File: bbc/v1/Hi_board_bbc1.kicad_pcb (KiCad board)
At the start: 2 copper layers, 55 x 61.1 mm, 15 parts, among them J1 sw-latch, J2 led-latch, J3 GLVMP, SW1 BSPD_RESET, SW2 IMD_RESET, SW3 BMS_RESET

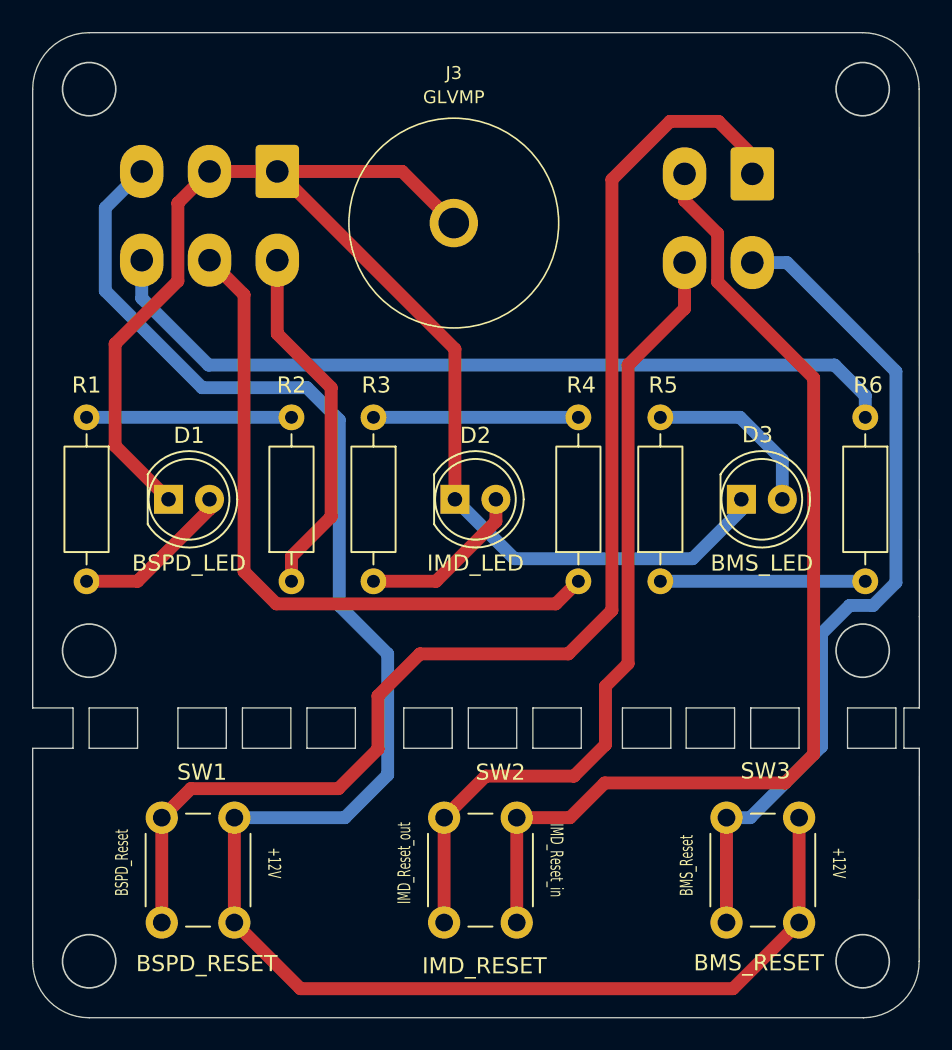
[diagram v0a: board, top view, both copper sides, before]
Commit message: Add files via upload
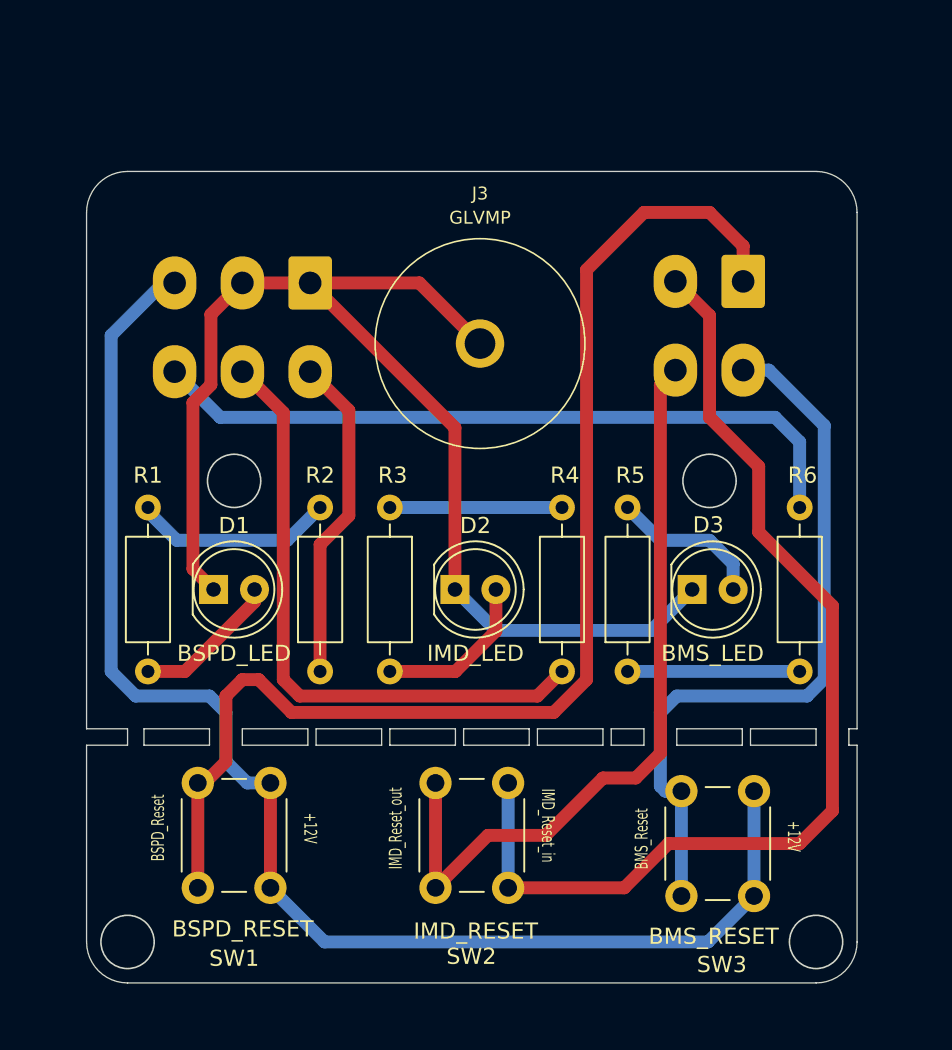
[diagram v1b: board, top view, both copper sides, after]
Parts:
- moved J3 7.64 mm to (141.2, 112.3)
- moved J2 7.20 mm to (130.7, 108.5)
- moved R6 6.91 mm to (161.0, 122.4)
- moved R1 6.76 mm to (120.6, 122.4)
- moved J1 6.69 mm to (157.5, 108.4)
- moved D3 6.37 mm to (154.4, 127.5)
- moved D1 6.25 mm to (124.7, 127.5)
- moved R5 5.95 mm to (150.4, 132.6)
- moved R2 5.86 mm to (131.3, 132.6)
- moved R3 5.68 mm to (135.6, 122.4)
- moved R4 5.68 mm to (146.3, 132.6)
- moved D2 5.59 mm to (139.7, 127.5)
- moved SW3 3.24 mm to (153.7, 146.5)
- moved SW1 3.10 mm to (123.7, 146.0)
- moved SW2 2.22 mm to (138.5, 146.0)
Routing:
- net +12V: track 111.4 -> 86.3 mm
- net 0: track 86.6 -> 76.6 mm
- net BMS_RESET: track 52.3 -> 45.7 mm
- net BMS_LED: track 51.0 -> 44.6 mm
- net IMD_LED: track 42.3 -> 38.5 mm
- net BSPD_RESET: track 80.6 -> 76.9 mm
- net IMD_RESET: track 50.3 -> 48.0 mm
- net Net-(R5-Pad1): track 12.7 -> 10.7 mm
- net Net-(R3-Pad1): track 12.7 -> 10.7 mm
- net BSPD_LED: track 22.3 -> 20.3 mm
- net Net-(D3-A): track 11.1 -> 9.58 mm
- net Net-(D1-A): track 10.1 -> 9.16 mm
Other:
- board size 55 x 61.1 mm -> 47.8 x 50.3 mm
